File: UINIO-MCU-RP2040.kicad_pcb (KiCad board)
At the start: 2 copper layers, 61.9 x 25.4 mm, 47 parts, among them J1 Conn_01x20_Pin, J2 Conn_01x20_Pin, J3 Conn_01x04_Pin, Q1 DMG1012T, SW1 ~{RESET}, SW2 ~{USB_BOOT}, U1 SGM2019-3.3YN5G, U2 SPI-25-Flash-WSON8, U3 RP2040, Y1 12MHz

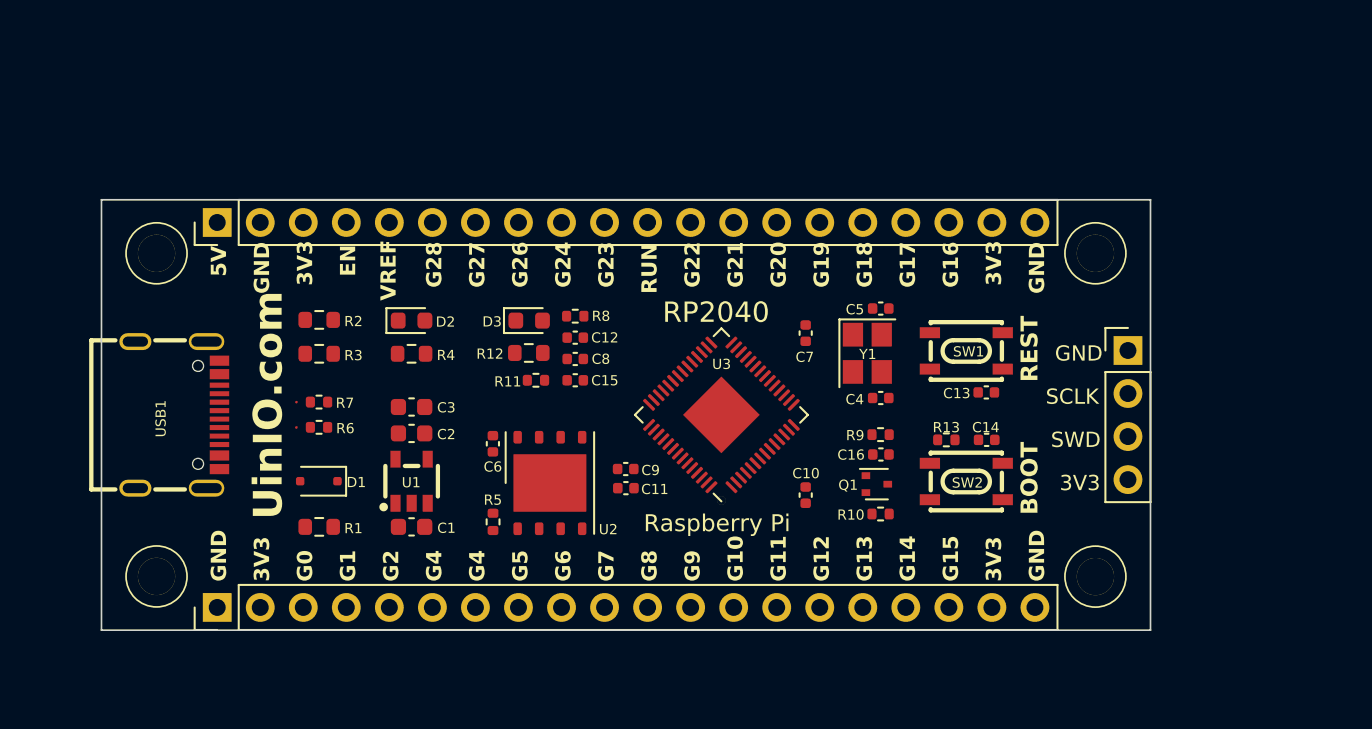
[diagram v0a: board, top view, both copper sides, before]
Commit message: Complete PCB wiring.
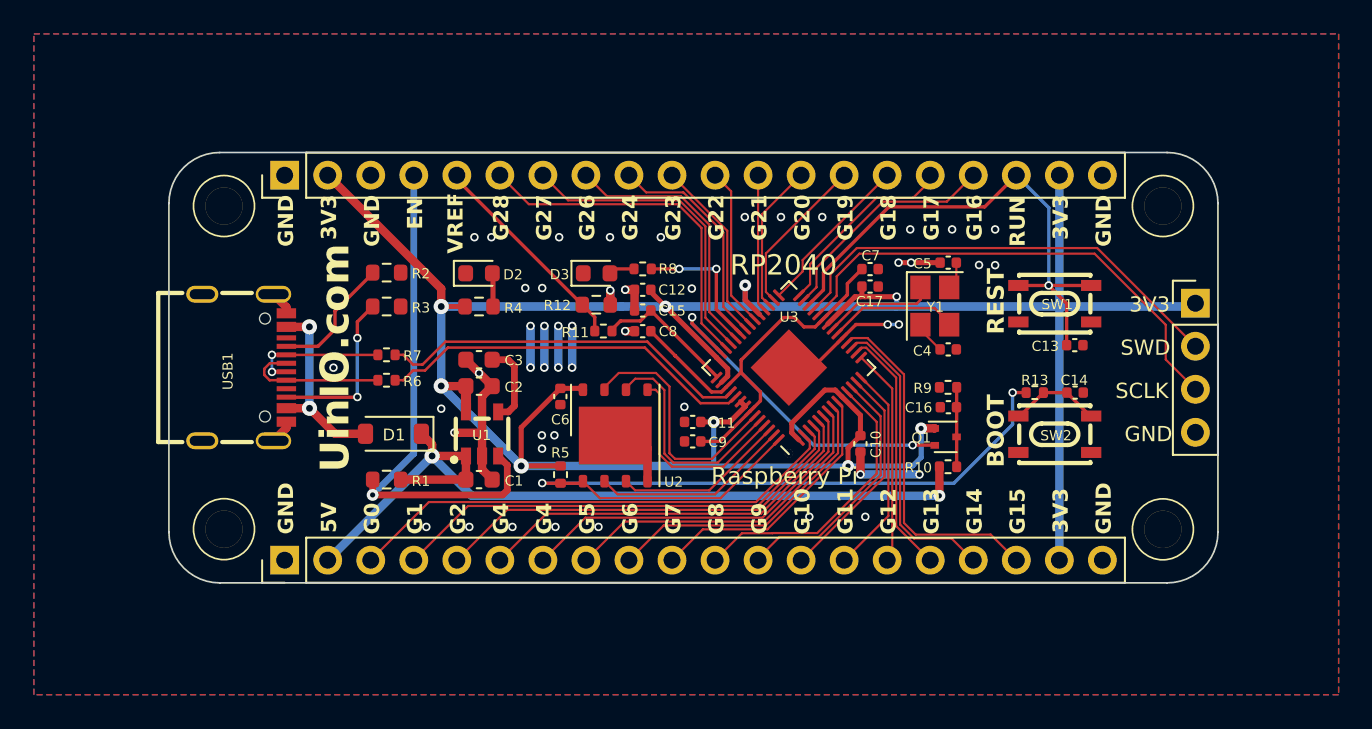
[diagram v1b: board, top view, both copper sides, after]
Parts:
- added C17: 0.1uF, Capacitor_SMD:C_0402_1005Metric, F.Cu at (157.2, 95.6)
- D1: footprint Diode_SMD:D_SOD-323F -> Diode_SMD:D_SOD-123
- moved R13 5.92 mm to (166.9, 101.8)
- moved SW2 5.92 mm to (168.1, 104.3)
- moved SW1 5.92 mm to (168.1, 96.6)
- moved C13 5.92 mm to (169.3, 99.0)
- moved C14 5.92 mm to (169.3, 101.8)
- moved C15 5.73 mm to (143.8, 97.0)
- moved C11 5.55 mm to (146.7, 103.5)
- moved C7 5.36 mm to (157.2, 94.5), turned to 0 degrees
- moved D1 5.22 mm to (129.0, 104.2)
- moved U1 5.01 mm to (134.3, 104.3)
- moved R11 4.93 mm to (141.4, 98.2)
- moved Q1 4.93 mm to (161.6, 104.4)
- moved C4 4.91 mm to (161.8, 99.3)
- moved R12 4.89 mm to (141.0, 96.6), turned to 180 degrees
- moved C12 4.88 mm to (143.8, 95.8)
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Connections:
- J1 pad 2: /VDD_3.3V -> /VDD_5V
- J2 pad 1: /VDD_5V -> GND
- J2 pad 11: /RUN -> /GPIO22
- J2 pad 12: /GPIO22 -> /GPIO21
- J2 pad 13: /GPIO21 -> /GPIO20
- J2 pad 14: /GPIO20 -> /GPIO19
- J2 pad 15: /GPIO19 -> /GPIO18
- J2 pad 16: /GPIO18 -> /GPIO17
- J2 pad 17: /GPIO17 -> /GPIO16
- J2 pad 18: /GPIO16 -> /RUN
- J2 pad 2: GND -> /VDD_3.3V
- J2 pad 3: /VDD_3.3V -> GND
- J3 pad 1: GND -> /VDD_3.3V
- J3 pad 4: /VDD_3.3V -> GND
- U3 pad 24: Net-(J3-Pin_2) -> Net-(J3-Pin_3)
- U3 pad 25: Net-(J3-Pin_3) -> Net-(J3-Pin_2)
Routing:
- net /VDD_3.3V: track 0.00 -> 163.3 mm, vias 0 -> 10
- net /VDD_5V: track 0.00 -> 50.1 mm, vias 0 -> 2
- net /Boot_Select: track 0.00 -> 47.6 mm, vias 0 -> 2
- net GND: track 0.00 -> 41.3 mm, vias 0 -> 47
- net /RUN: track 0.00 -> 31.6 mm, vias 0 -> 1
- net /LDO_EN: track 0.00 -> 31.0 mm, vias 0 -> 1
- net /GPIO0: track 0.00 -> 29.6 mm
- net Net-(J3-Pin_3): track 0.00 -> 28.9 mm
- net /GPIO1: track 0.00 -> 27.6 mm
- net Net-(J3-Pin_2): track 0.00 -> 27.1 mm
- net /GPIO2: track 0.00 -> 25.7 mm
- net +1V1: track 0.00 -> 24.9 mm
- net /GPIO3: track 0.00 -> 23.7 mm
- net /USB_Data+: track 0.00 -> 22.4 mm
- net /USB_Data-: track 0.00 -> 22.1 mm
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- added copper zone on B.Cu, net GND
- added copper zone on F.Cu, net GND
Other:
- outline, holes or cut-outs redrawn
- board text added: "UINIO-MCU-RP2040"
- board text added: "Version 1.0.0"
